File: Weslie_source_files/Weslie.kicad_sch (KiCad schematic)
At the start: 5 parts

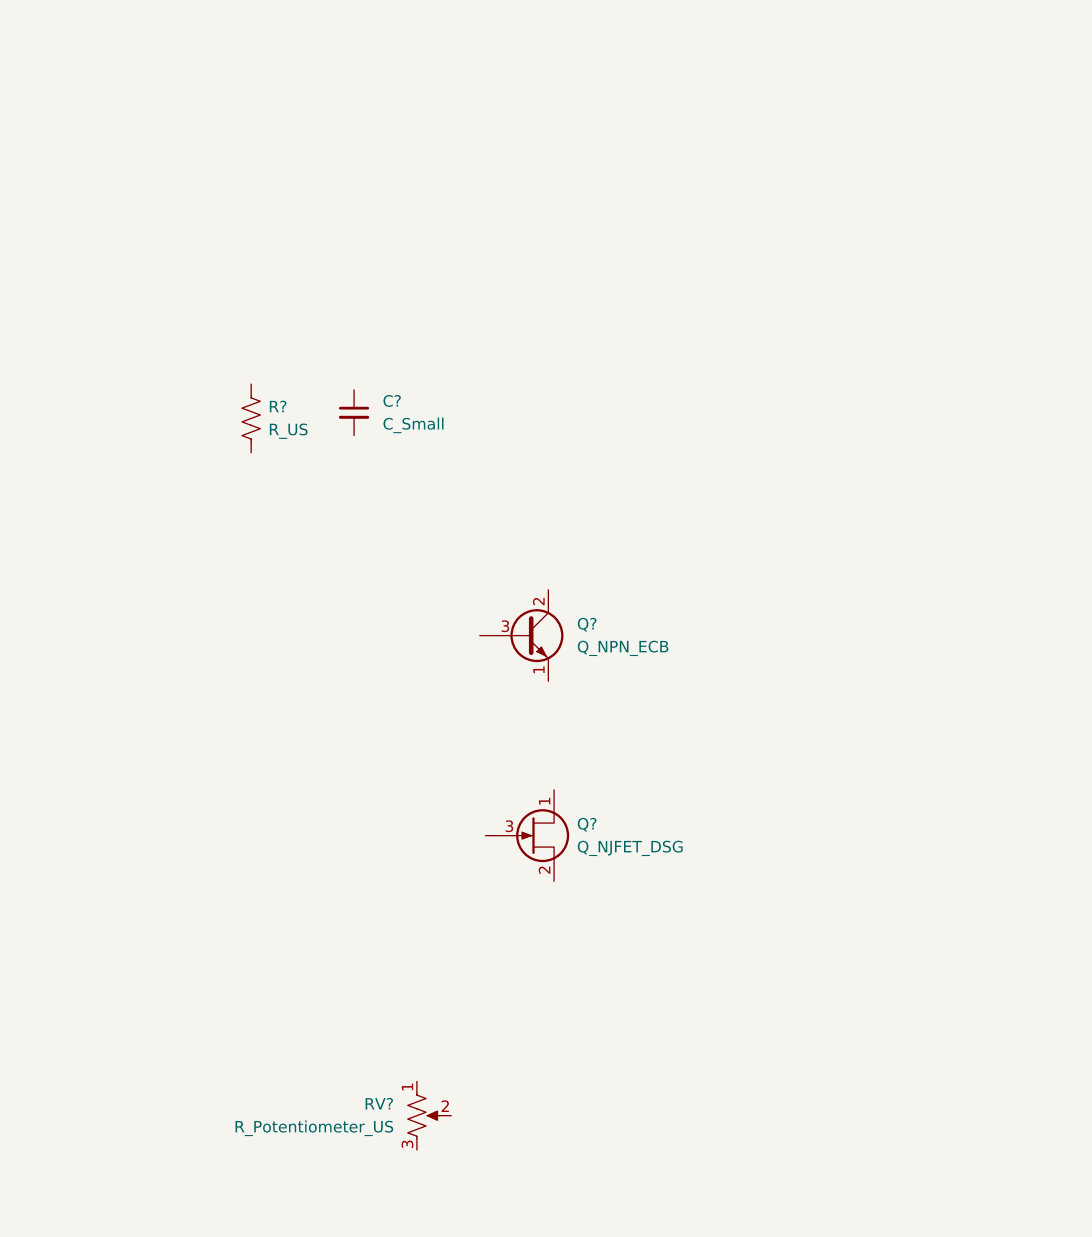
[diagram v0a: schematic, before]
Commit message: Schematic
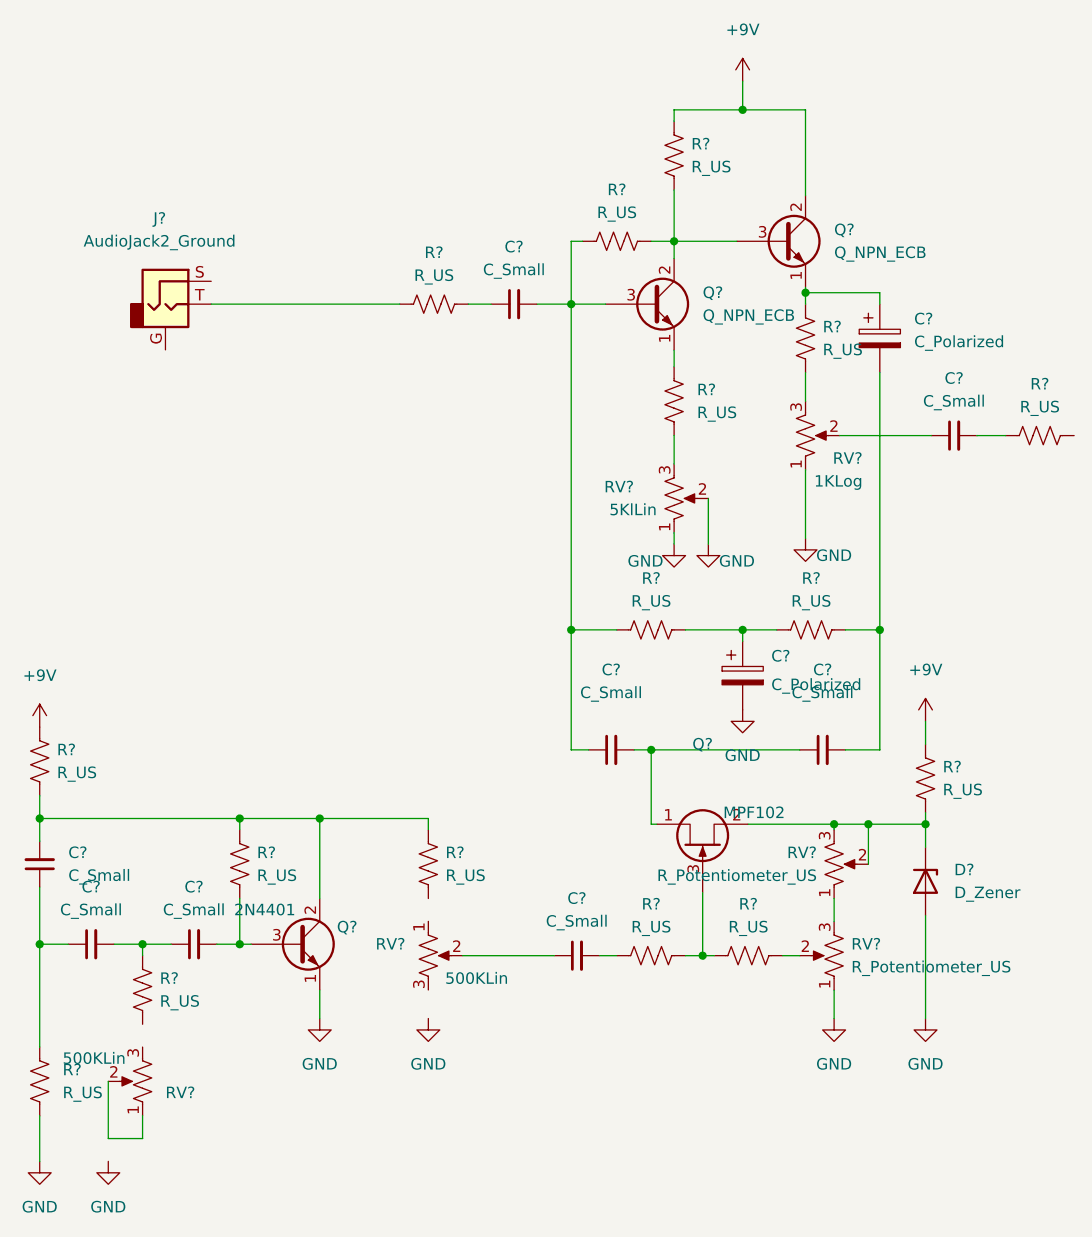
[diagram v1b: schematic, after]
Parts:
- added C? (x7): C_Small, symbol Device:C_Small
- added C? (x2): C_Polarized, symbol Device:C_Polarized
- added D?: D_Zener, symbol Device:D_Zener
- added J?: AudioJack2_Ground, symbol Connector:AudioJack2_Ground
- added Q?: Q_NPN_ECB, symbol Device:Q_NPN_ECB
- added Q?: 2N4401, symbol Device:Q_NPN_ECB
- added R? (x15): R_US, symbol Device:R_US
- added RV? (x2): 500KLin, symbol Device:R_Potentiometer_US
- added RV? (x2): R_Potentiometer_US, symbol Device:R_Potentiometer_US
- added RV?: 5KlLin, symbol Device:R_Potentiometer_US
- Q?: value Q_NJFET_DSG -> MPF102
- RV?: value R_Potentiometer_US -> 1KLog
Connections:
- net at C?.1: now also R?.2
- net at C?.2: now also Q?.3 (B), C?.1, R?.1, R?.1
- net GND: now reaches RV?.1
- net GND: now also C?.2, D?.2 (A), Q?.1 (E), R?.1, RV?.1, RV?.1, RV?.2
- net at RV?.2: now also C?.1
- net at RV?.3: now also R?.1
- net at R?.1: now also J?.T
- net at Q?.1 (E): now also R?.2
- net at Q?.2 (C): now also Q?.3 (B), R?.1, R?.2
- net at Q?.1 (D): now also C?.1, C?.2
- net at Q?.2 (S): now also D?.1 (K), R?.1, RV?.2, RV?.3
- net at Q?.3 (G): now also R?.1, R?.2
- new net: RV?.1, RV?.2
- new net: C?.2, R?.1 (x2)
- new net: C?.1, Q?.1 (E), R?.2
- new net: C?.2, C?.2, R?.2
- new net: RV?.1, RV?.3
- new net: C?.1, R?.1, R?.2
- new net: R?.1, RV?.3
- new net: C?.1, C?.1, R?.2
- new net: C?.2, Q?.2 (C), R?.1, R?.2, R?.2
- new net: C?.1, RV?.2
- new net: C?.1, C?.2, R?.2
- new net: C?.2, Q?.3 (B), R?.1
- new net: R?.2, RV?.2
- new net +9V: Q?.2 (C), R?.2, R?.2, R?.2
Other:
- moved on the sheet: C?, Q?, R?, RV?
